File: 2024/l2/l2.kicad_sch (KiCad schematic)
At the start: 20 parts, among them J1 Conn_01x04, J2 Conn_01x02, J3 Conn_01x04, U5 DEV-15583

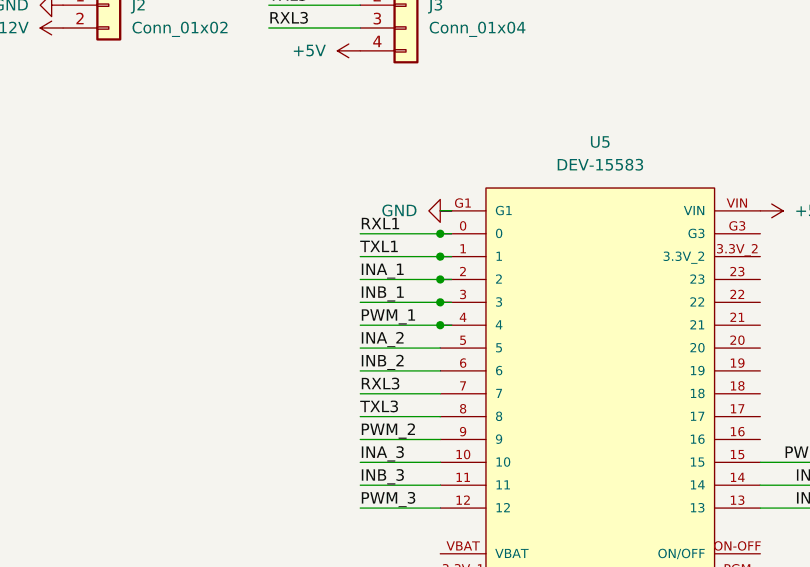
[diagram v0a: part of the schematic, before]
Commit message: 16/8 final
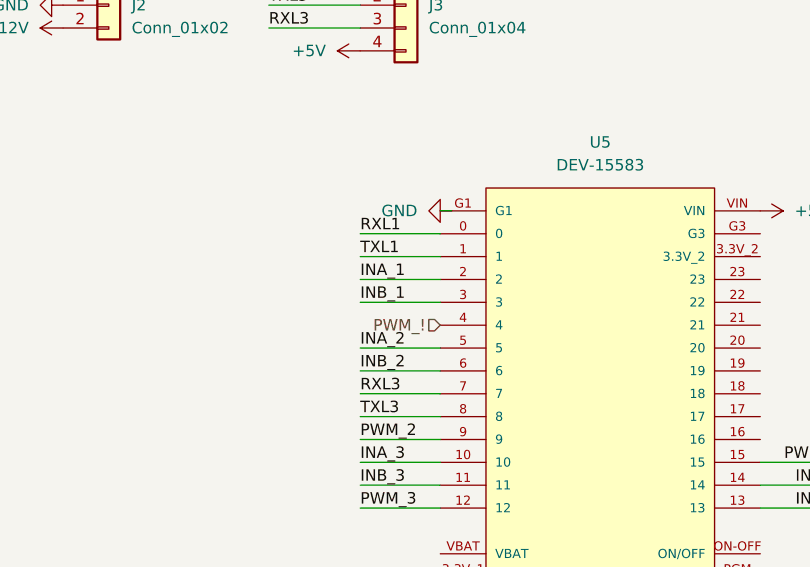
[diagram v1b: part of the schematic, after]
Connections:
- net PWM_1 renamed PWM_!
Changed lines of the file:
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@@
 	(generator_version "8.0")
 	(paper "A4")
-	(junction
-		(at 203.2 52.07)
-		(diameter 0)
-		(color 0 0 0 0)
-	)
-	(junction
-		(at 203.2 49.53)
-		(diameter 0)
-		(color 0 0 0 0)
-	)
-	(junction
-		(at 203.2 46.99)
-		(diameter 0)
-		(color 0 0 0 0)
-	)
-	(junction
-		(at 203.2 57.15)
-		(diameter 0)
-		(color 0 0 0 0)
-	)
-	(junction
-		(at 203.2 54.61)
-		(diameter 0)
-		(color 0 0 0 0)
-	)
 	(no_connect
 		(at 222.25 139.7)
@@
 	(wire
 		(pts
-			(xy 204.47 49.53) (xy 203.2 49.53)
-		)
-		(stroke
-			(width 0)
-			(type default)
-		)
-	)
-	(wire
-		(pts
 			(xy 247.65 77.47) (xy 238.76 77.47)
 		)
@@
 	(wire
 		(pts
-			(xy 204.47 57.15) (xy 203.2 57.15)
-		)
-		(stroke
-			(width 0)
-			(type default)
-		)
-	)
-	(wire
-		(pts
-			(xy 204.47 54.61) (xy 203.2 54.61)
-		)
-		(stroke
-			(width 0)
-			(type default)
-		)
-	)
-	(wire
-		(pts
 			(xy 194.31 54.61) (xy 203.2 54.61)
 		)
@@
 	(wire
 		(pts
-			(xy 204.47 46.99) (xy 203.2 46.99)
-		)
-		(stroke
-			(width 0)
-			(type default)
-		)
-	)
-	(wire
-		(pts
 			(xy 194.31 67.31) (xy 203.2 67.31)
 		)
@@
 		(pts
 			(xy 194.31 77.47) (xy 203.2 77.47)
-		)
-		(stroke
-			(width 0)
-			(type default)
-		)
-	)
-	(wire
-		(pts
-			(xy 204.47 52.07) (xy 203.2 52.07)
-		)
-		(stroke
-			(width 0)
-			(type default)
-		)
-	)
-	(wire
-		(pts
-			(xy 194.31 57.15) (xy 203.2 57.15)
 		)
 		(stroke
@@
 		)
 	)
-	(label "PWM_1"
-		(at 194.31 57.15 0)
-		(fields_autoplaced yes)
-		(effects
-			(font
-				(size 1.27 1.27)
-			)
-			(justify left bottom)
-		)
-	)
 	(label "INB_2"
 		(at 194.31 62.23 0)
@@
 		)
 	)
+	(hierarchical_label "PWM_!"
+		(shape input)
+		(at 203.2 57.15 180)
+		(fields_autoplaced yes)
+		(effects
+			(font
+				(size 1.27 1.27)
+			)
+			(justify right)
+		)
+	)

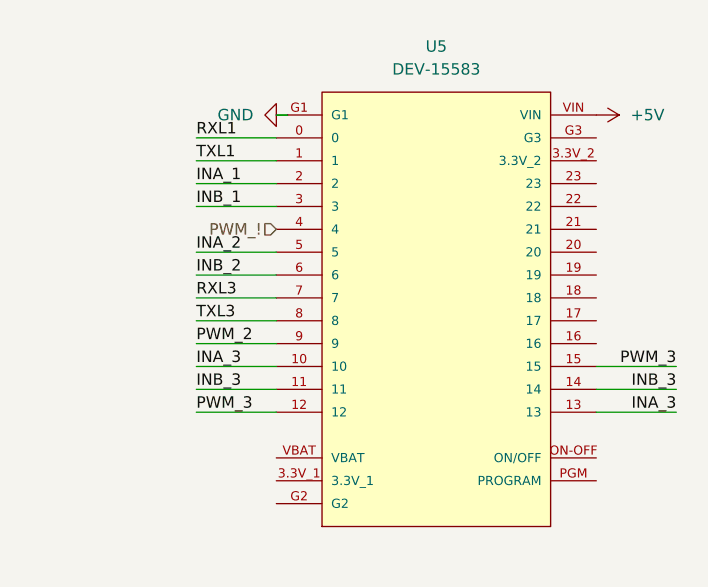
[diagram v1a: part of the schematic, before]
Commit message: 21/8 final
about 10% done l2 pcb
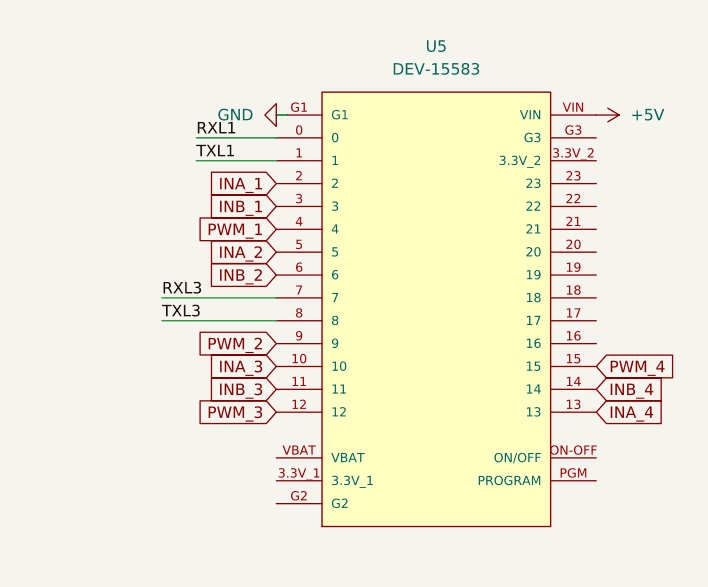
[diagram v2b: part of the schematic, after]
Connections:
- net INA_3: no longer U5.13
- net INB_3: no longer U5.14
- net PWM_3: no longer U5.15
- net PWM_! renamed PWM_1
- new net INA_4: U5.13
- new net INB_4: U5.14
- new net PWM_4: U5.15
